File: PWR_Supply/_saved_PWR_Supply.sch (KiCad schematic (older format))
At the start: 0 parts

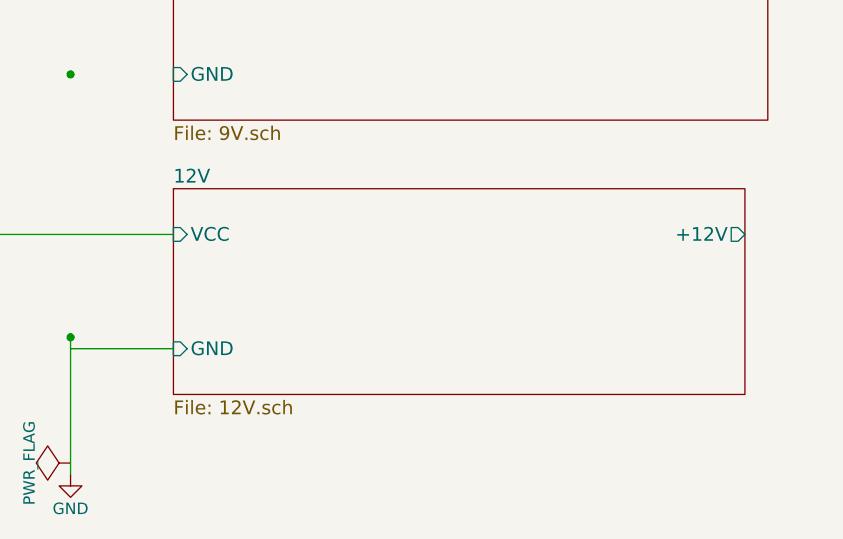
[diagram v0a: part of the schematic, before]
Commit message: single_amp
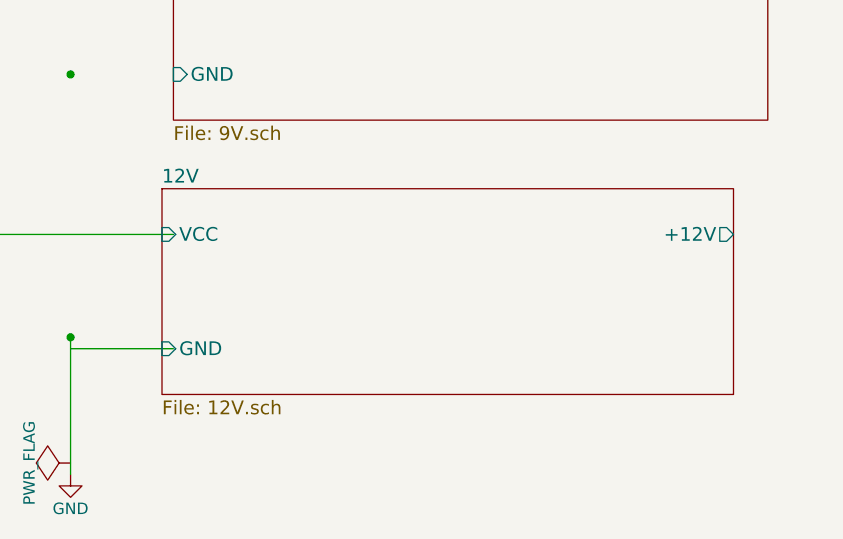
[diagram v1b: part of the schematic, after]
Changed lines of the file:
@@
 $EndSheet
 $Sheet
-S 1650 6200 2500 900
+S 1600 6200 2500 900
 U 58D2C80A
 F0 "12V" 60
 F1 "12V.sch" 60
-F2 "+12V" O R 4150 6400 60
-F3 "GND" I L 1650 6900 60
-F4 "VCC" I L 1650 6400 60
+F2 "+12V" O R 4100 6400 60
+F3 "GND" I L 1600 6900 60
+F4 "VCC" I L 1600 6400 60
 $EndSheet
 $Comp
